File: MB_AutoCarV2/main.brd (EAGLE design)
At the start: 224.8 x 121.6 mm, 44 parts, among them K1 CQ1-12V, K2 CQ1-12V, K3 CQ1-12V, K4 CQ1-12V, Q1 PN2222, Q2 PN2222, Q3 PN2222, Q4 PN2222, U1 ARDUINO-MEGAFULL

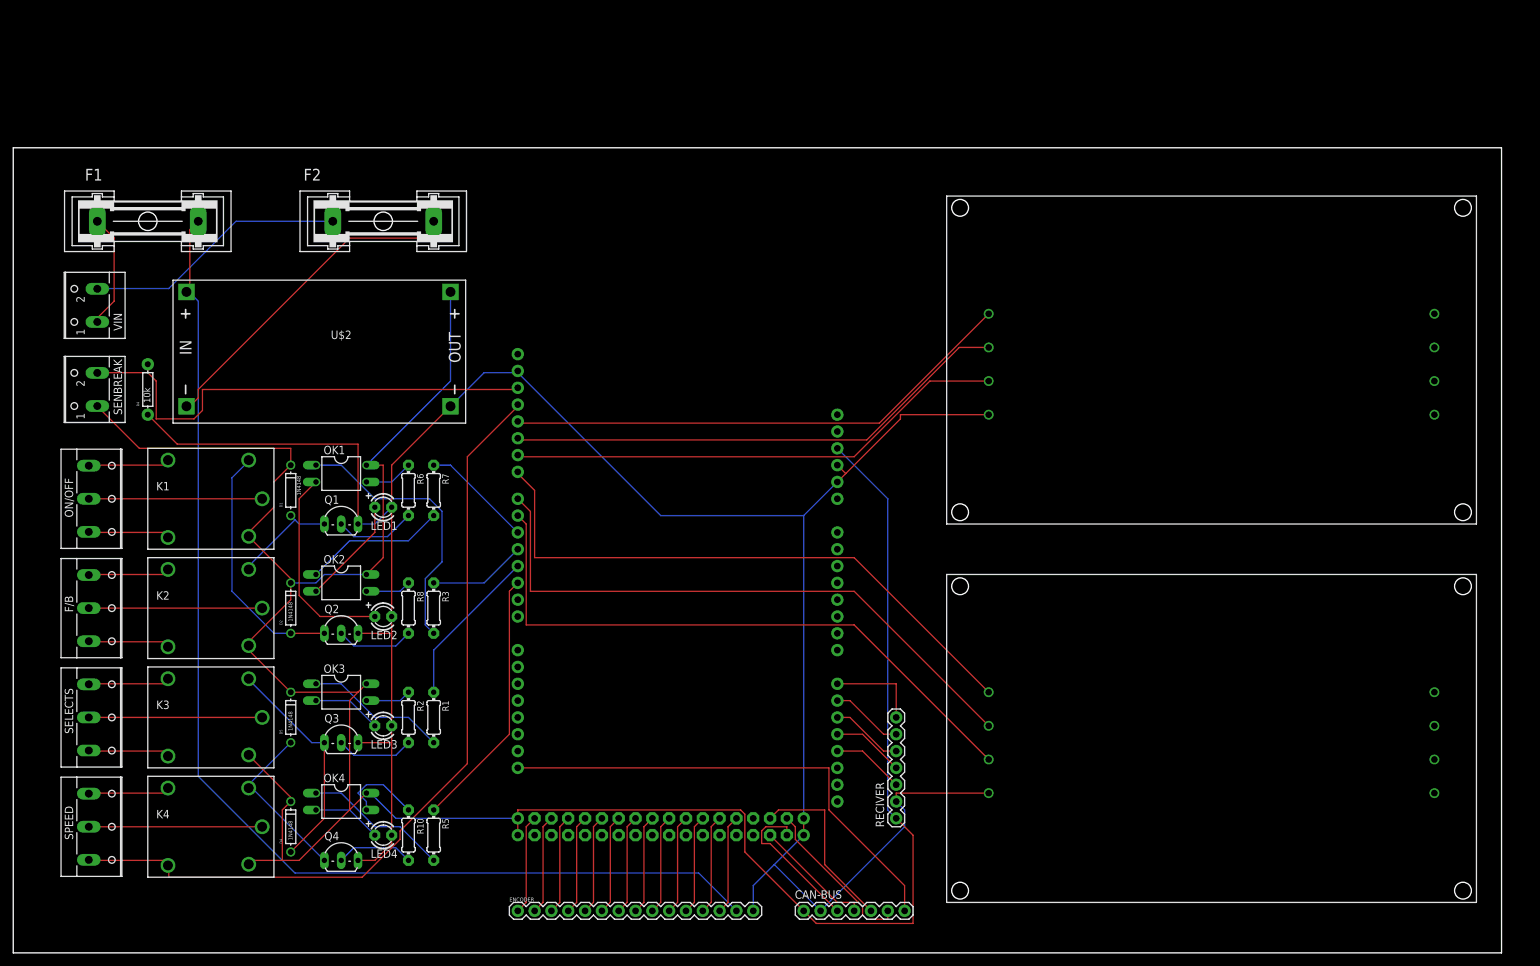
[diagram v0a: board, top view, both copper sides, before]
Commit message: update
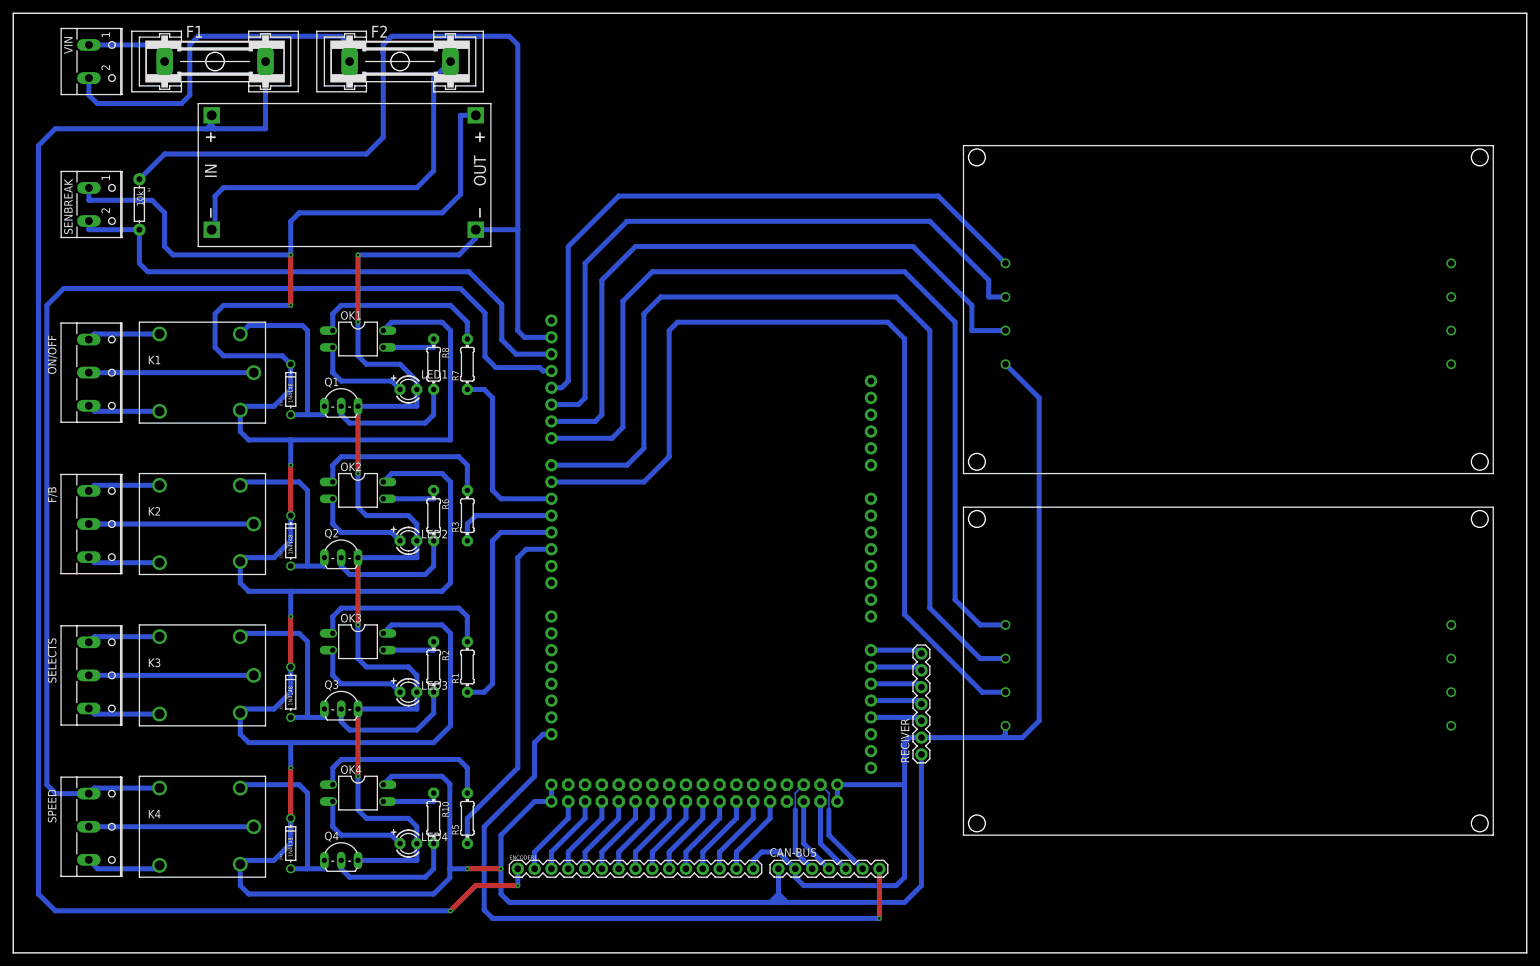
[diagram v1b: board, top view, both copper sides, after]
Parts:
- removed D1, D2, D4, D5: 1N4148, adafruit:DO-1N4148
- removed ENCODER: (no value), SparkFun-Connectors:1X15
- added D11, D22, D33, D44: 1N4148, adafruit:DO-1N4148
- added ENCODER1: (no value), SparkFun-Connectors:1X15
- moved R8 37.0 mm to (63.5, 88.9)
- moved VIN 36.9 mm to (12.7, 134.6), turned to 270 degrees
- moved R4 28.0 mm to (19.1, 113.0), turned to 270 degrees
- moved SENBREAK 28.0 mm to (12.7, 113.0), turned to 270 degrees
- moved U$2 26.9 mm to (52.1, 118.1)
- moved F1 26.2 mm to (30.5, 134.6)
- moved F2 24.3 mm to (58.4, 134.6)
- moved OK1 20.5 mm to (52.1, 92.7)
- moved R7 19.7 mm to (68.6, 88.9), turned to 90 degrees
- moved K1 19.1 mm to (29.2, 87.6)
- moved ON/OFF 19.0 mm to (12.7, 87.6)
- moved LED1 18.2 mm to (59.7, 85.1)
- moved Q1 17.8 mm to (49.5, 83.8)
- moved R3 14.9 mm to (68.6, 66.0), turned to 90 degrees
- moved OK2 14.2 mm to (52.1, 69.8)
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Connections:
- removed net D22: ENCODER.1, U1.22
- removed net D24: ENCODER.2, U1.24
- removed net D26: ENCODER.3, U1.26
- removed net D28: ENCODER.4, U1.28
- removed net D30: ENCODER.5, U1.30
- removed net D32: ENCODER.6, U1.32
- removed net D34: ENCODER.7, U1.34
- removed net D36: ENCODER.8, U1.36
- removed net D38: ENCODER.9, U1.38
- removed net D40: ENCODER.10, U1.40
- removed net D42: ENCODER.11, U1.42
- removed net D44: ENCODER.12, U1.44
- removed net D46: ENCODER.13, U1.46
- removed net D48: U1.48
- removed net N$1: K4.NO, SPEED.1
- new net D23: ENCODER1.2, U1.23
- new net D25: ENCODER1.3, U1.25
- new net D27: ENCODER1.4, U1.27
- new net D29: ENCODER1.5, U1.29
- new net D31: ENCODER1.6, U1.31
- new net D33: ENCODER1.7, U1.33
- new net D35: ENCODER1.8, U1.35
- new net D37: ENCODER1.9, U1.37
- new net D39: ENCODER1.10, U1.39
- new net D41: ENCODER1.11, U1.41
- new net D43: ENCODER1.12, U1.43
- new net D45: ENCODER1.13, U1.45
- new net D47: ENCODER1.14, U1.47
- new net D49: U1.49
- new net N$13: K4.NC, SPEED.3
- net !CS: now also CAN-BUS.5; no longer CAN-BUS.3
- net 22: now also D11.A, Q1.C; no longer D2.A, Q2.C
- net 3: now also D33.A; no longer D4.A
- net 6: now also D44.A; no longer D5.A
- net D12PWM: now also K4.NO, SPEED.1; no longer K4.NC, SPEED.3
- net GND: now also ENCODER1.15; no longer ENCODER.15, U1.GND@0, U1.GND@1
- net GND-: now also D22.A, Q2.C; no longer D1.A, Q1.C
- net INS: now also OK2.1; no longer OK1.1
- net INSS: now also OK1.1; no longer OK2.1
- net LED: now also OK2.2; no longer OK1.2
- net LEDS: now also OK1.2; no longer OK2.2
- net MISO: now also CAN-BUS.3; no longer CAN-BUS.5
- net N$12: now also Q2.B; no longer Q1.B
- net N$20: now also Q1.B; no longer Q2.B
- net N$22: now also OK1.3; no longer OK2.3
- net OTP: now also OK2.3; no longer OK1.3
- net VCC: now also D11.C, D22.C, D33.C, D44.C; no longer D1.C, D2.C, D4.C, D5.C, U1.5V@0
- net VIN: now also ENCODER1.1; no longer ENCODER.14
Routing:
- net VCC: track 389.5 -> 582.4 mm, vias 0 -> 7
- net GND: track 349.1 -> 446.4 mm, vias 0 -> 5
- net VIN: track 175.2 -> 239.3 mm, vias 0 -> 2
- net D12PWM: track 124.8 -> 176.6 mm
- net D8PWM: track 91.0 -> 136.8 mm
- net D7PWM: track 92.4 -> 138.2 mm
- net D6PWM: track 95.3 -> 137.3 mm
- net INT: track 73.3 -> 99.2 mm, vias 0 -> 1
- net D9PWM: track 76.1 -> 98.9 mm
- net D10PWM: track 77.2 -> 98.2 mm
- net D11PWM: track 78.2 -> 96.7 mm
- net LED: track 30.9 -> 15.0 mm
- net D42: track 15.0 -> 0.00 mm
- net D38: track 15.0 -> 0.00 mm
- net D28: track 15.0 -> 0.00 mm
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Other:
- board size 224.8 x 121.6 mm -> 228.6 x 141.9 mm
